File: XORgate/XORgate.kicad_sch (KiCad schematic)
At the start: 0 parts

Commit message: update
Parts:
- added J1, J2, J3, J4: Conn_01x02_Pin, Connector_PinHeader_2.00mm:PinHeader_1x02_P2.00mm_Vertical, symbol Connector:Conn_01x02_Pin
- added U1, U2: ~, Package_DIP:DIP-14_W7.62mm, symbol Transistor_FET:CD4007
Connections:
- new net: U1.1 (S), U1.11 (S)
- new net: U1.2 (D), U2.2 (D)
- new net: J1.1 (Pin_1), U1.3 (G), U1.3 (G), U1.6 (G), U1.6 (G)
- new net: J2.1 (Pin_1), U2.10 (G), U2.10 (G), U2.6 (G), U2.6 (G)
- new net: U2.1 (S), U2.11 (S)
- new net: J3.1 (Pin_1), U1.12 (D), U1.9 (D), U2.12 (D), U2.9 (D)
- new net: U1.5 (D), U2.12 (S)
- new net: U1.10 (G), U1.13 (S), U1.8 (D), U2.3 (G)
- new net: U1.10 (G), U2.13 (S), U2.3 (G), U2.8 (D)
- new net: J4.1 (Pin_1), U1.14 (D), U2.14 (D)
- new net: U1.12 (S), U2.5 (D)
- new net: U1.4 (S), U2.4 (S)
- new net GND: J1.2 (Pin_2), J2.2 (Pin_2), J3.2 (Pin_2), J4.2 (Pin_2), U1.7 (S), U2.7 (S)

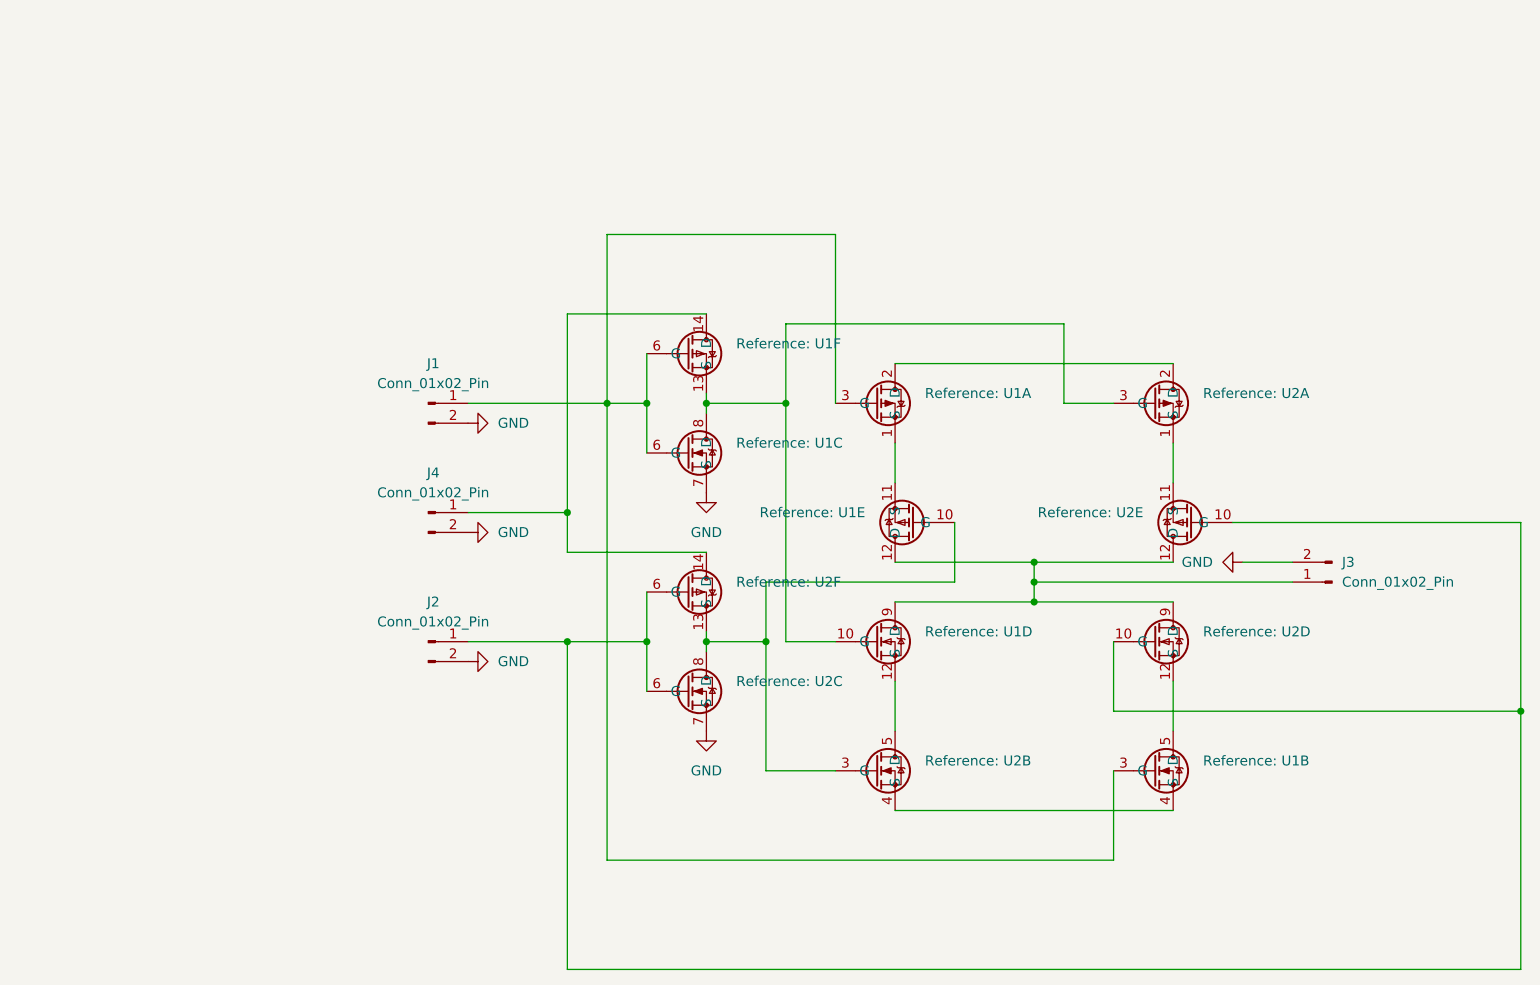
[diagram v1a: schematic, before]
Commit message: update
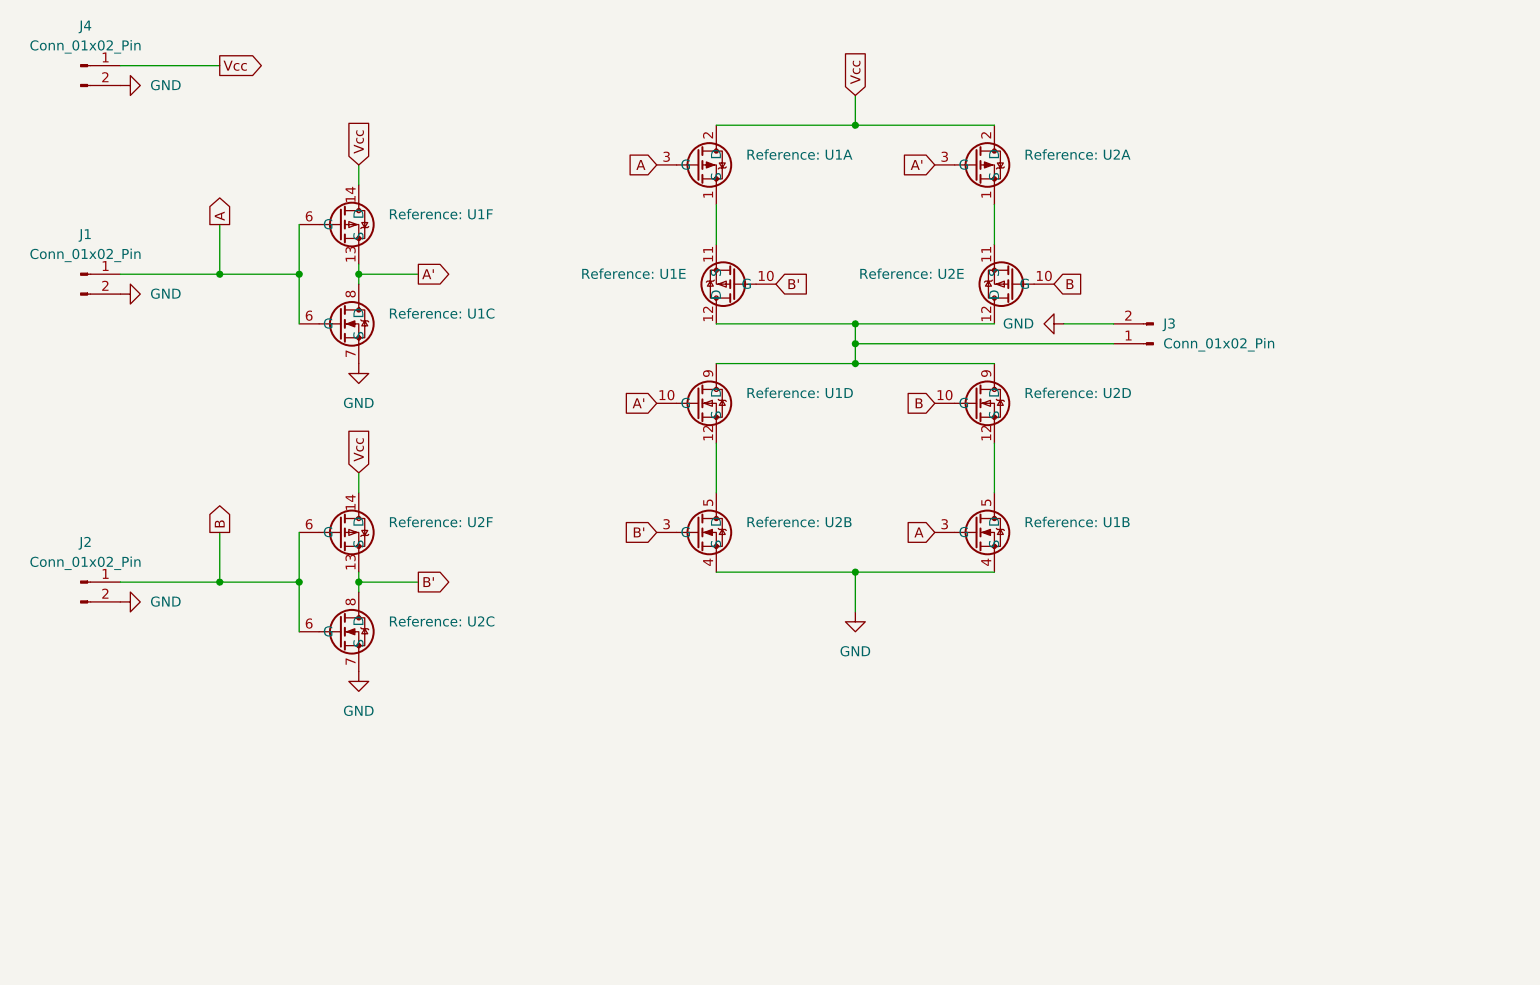
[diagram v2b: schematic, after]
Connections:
- net GND: now also U1.4 (S), U2.4 (S)
- net Vcc: now reaches U1.2 (D), U2.2 (D)
- net Vcc: now also J4.1 (Pin_1), U1.14 (D), U2.14 (D)
- net A: now reaches J1.1 (Pin_1), U1.3 (G), U1.3 (G), U1.6 (G), U1.6 (G)
- net B: now reaches J2.1 (Pin_1), U2.10 (G), U2.10 (G), U2.6 (G), U2.6 (G)
- net A': now reaches U1.10 (G), U1.13 (S), U1.8 (D), U2.3 (G)
- net B': now reaches U1.10 (G), U2.13 (S), U2.3 (G), U2.8 (D)
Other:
- company: (none) -> McMaster University ECE
- title: (none) -> XOR Gate Constructed with 12 MOSFETs Using 2 CD4007 ICs
- moved on the sheet: J1, J2, J3, J4, Reference: U1A, Reference: U1B, Reference: U1C, Reference: U1D, Reference: U1E, Reference: U1F, Reference: U2A, Reference: U2B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
